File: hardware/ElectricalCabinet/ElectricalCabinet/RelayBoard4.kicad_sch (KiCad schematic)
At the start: 0 parts

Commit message: Further wiring updates
Populated 6100 Bus
Corrected number of relay boards
Added 110v outputs to relay boards and noted light positon
Uploaded light scheme to documents folder
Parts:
- added C4: 0.1uF, Capacitor_SMD:C_0805_2012Metric, symbol Device:C
- added D25, D26, D27, D28, D29, D30, D31, D32: LED, LED_SMD:LED_0805_2012Metric, symbol Device:LED
- added J8: Screw_Terminal_01x06, TerminalBlock:TerminalBlock_MaiXu_MX126-5.0-06P_1x06_P5.00mm, symbol Connector:Screw_Terminal_01x06
- added J9: Screw_Terminal_01x09, TerminalBlock:TerminalBlock_MaiXu_MX126-5.0-09P_1x09_P5.00mm, symbol Connector:Screw_Terminal_01x09
- added K25, K26, K27, K28, K29, K30, K31, K32: G3MB-202P DC5, TrafficLightLibrary:G3MB_202P_DC5, symbol TrafficLightLibrary:G3MB-202P_DC5
- added R25, R26, R27, R28, R29, R30, R31, R32: 1kΩ, Resistor_SMD:R_0805_2012Metric, symbol Device:R
- added U5: TPIC6B595N, TrafficLightLibrary:TPIC6B595N, symbol TrafficLightLibrary:TPIC6B595N
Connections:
- new net: D25.1 (K), R25.1
- new net: D25.2 (A), D26.2 (A), D27.2 (A), D28.2 (A), D29.2 (A), D30.2 (A), D31.2 (A), D32.2 (A), K25.3, K26.3, K27.3, K28.3, K29.3, K30.3, K31.3, K32.3
- new net: J9.1 (Pin_1), K25.2
- new net: J9.2 (Pin_2), K26.2
- new net: J9.3 (Pin_3), K27.2
- new net: J9.4 (Pin_4), K28.2
- new net: J9.5 (Pin_5), K29.2
- new net: J9.6 (Pin_6), K30.2
- new net: J9.7 (Pin_7), K31.2
- new net: J9.8 (Pin_8), K32.2
- new net: J9.9 (Pin_9), K25.1, K26.1, K27.1, K28.1, K29.1, K30.1, K31.1, K32.1
- new net: K30.4, R30.2, U5.15 (DRAIN5)
- new net: C4.1, J8.2 (Pin_2), U5.10 (GND), U5.11 (GND), U5.19 (GND), U5.9 (~{G})
- new net: J8.4 (Pin_4), U5.12 (RCK)
- new net: J8.3 (Pin_3), U5.13 (SRCK)
- new net: K29.4, R29.2, U5.14 (DRAIN4)
- new net: K31.4, R31.2, U5.16 (DRAIN6)
- new net: K32.4, R32.2, U5.17 (DRAIN7)
- new net: J8.1 (Pin_1), U5.18 (SEROUT)
- new net: C4.2, J8.6 (Pin_6), U5.2 (VCC), U5.8 (~{SRCLR})
- new net: K25.4, R25.2, U5.4 (DRAIN0)
- new net: K26.4, R26.2, U5.5 (DRAIN1)
- new net: K27.4, R27.2, U5.6 (DRAIN2)
- new net: K28.4, R28.2, U5.7 (DRAIN3)
- new net: D27.1 (K), R27.1
- new net: D26.1 (K), R26.1
- new net: D31.1 (K), R31.1
- new net: D30.1 (K), R30.1
- new net: D32.1 (K), R32.1
- new net: D29.1 (K), R29.1
- new net: D28.1 (K), R28.1
- new net SERIN: J8.5 (Pin_5), U5.3 (SERIN)
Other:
- note added: "RELAY MODULE 4"

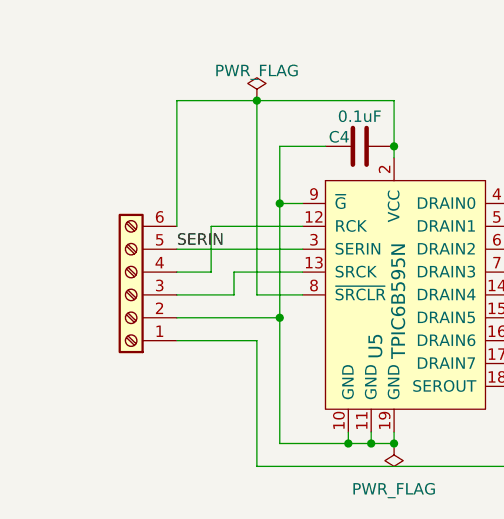
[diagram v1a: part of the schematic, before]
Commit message: Electrical Cabinet done
Electrical Cabinet done, let me know if there are any changes or mistakes.
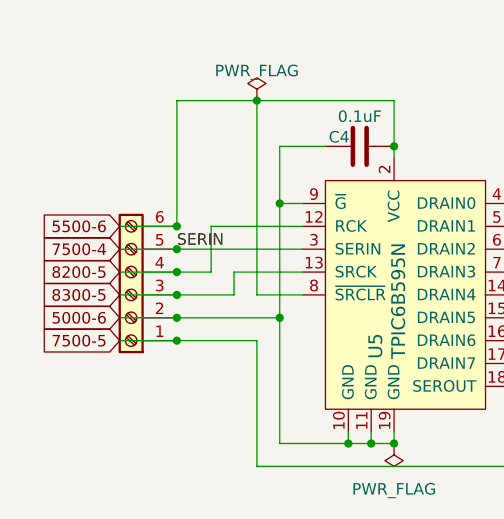
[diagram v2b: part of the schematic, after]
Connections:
- net 5000-6: now reaches C4.1, J8.2 (Pin_2), U5.10 (GND), U5.11 (GND), U5.19 (GND), U5.9 (~{G})
- net 8200-5: now reaches J8.4 (Pin_4), U5.12 (RCK)
- net 8300-5: now reaches J8.3 (Pin_3), U5.13 (SRCK)
- net 7500-5: now reaches J8.1 (Pin_1), U5.18 (SEROUT)
- net 5500-6: now reaches C4.2, J8.6 (Pin_6), U5.2 (VCC), U5.8 (~{SRCLR})
- net SERIN renamed 7500-4
